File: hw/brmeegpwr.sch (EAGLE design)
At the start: 9 parts, among them IC1 MAX639, IC2 MAX639, IC3 MAX639

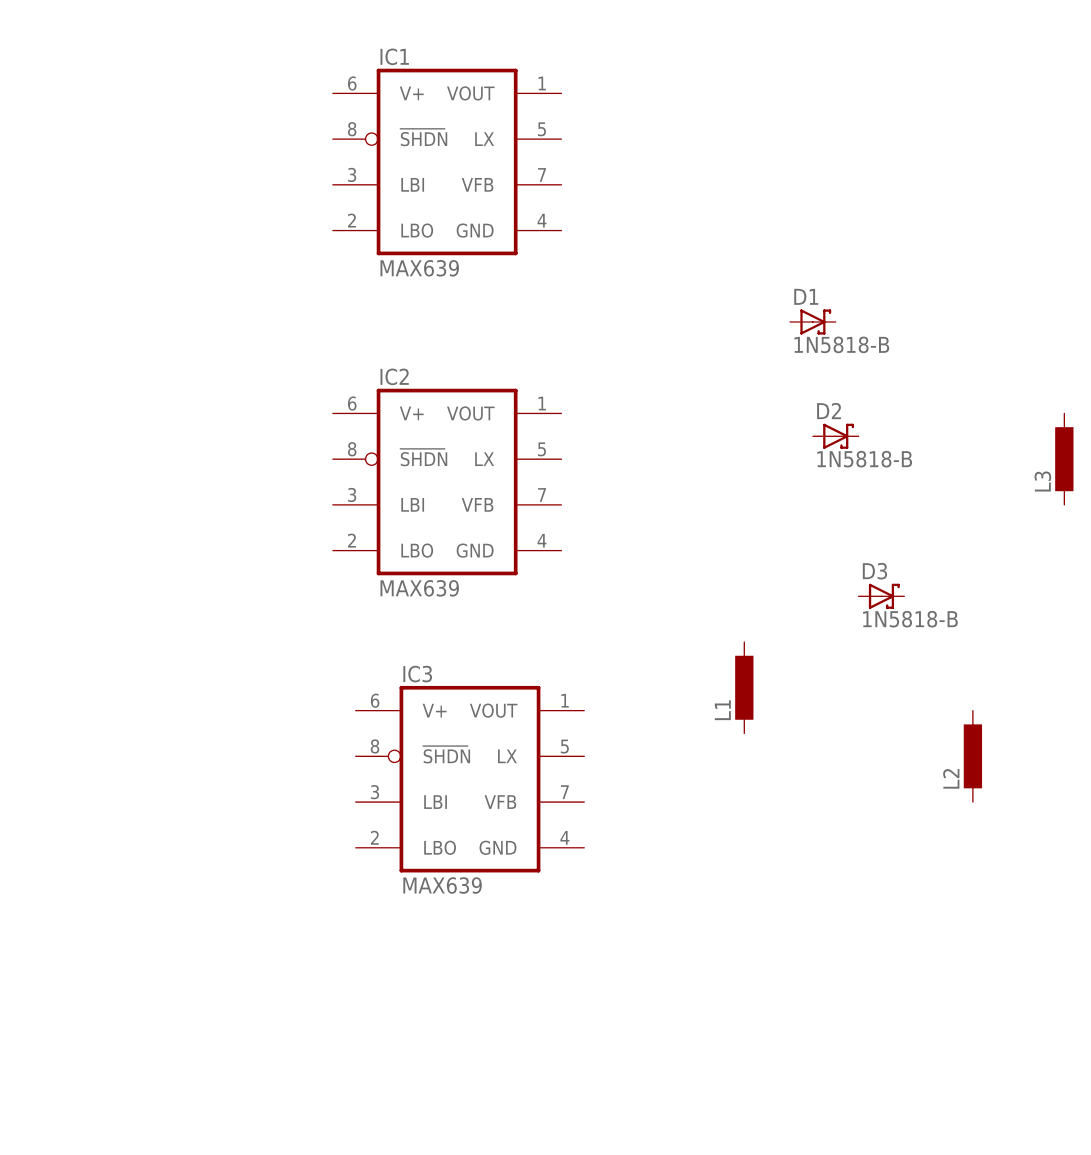
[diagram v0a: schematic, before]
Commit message: power supplies
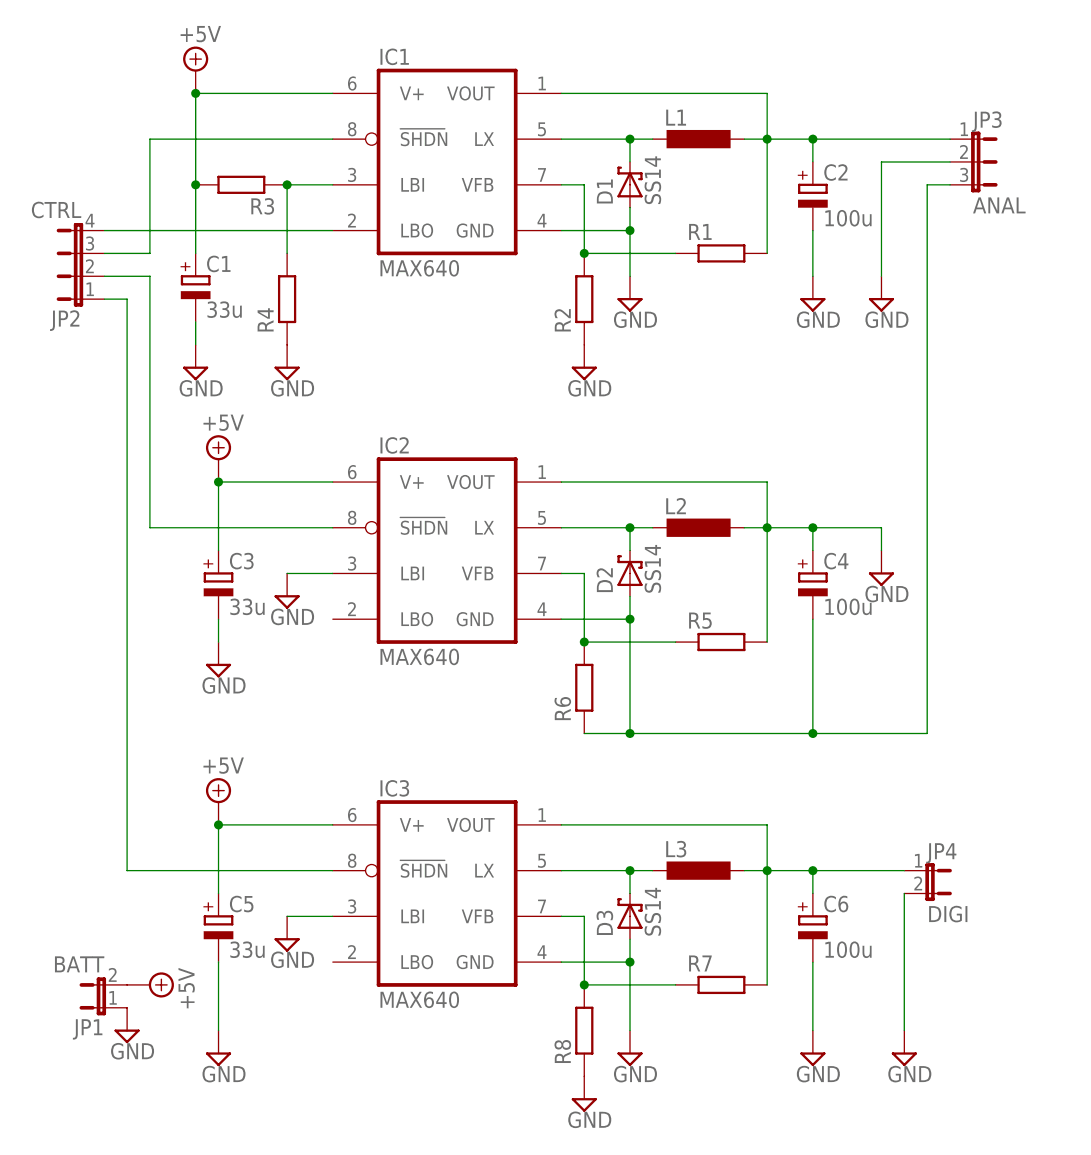
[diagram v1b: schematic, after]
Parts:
- added C1, C3, C5: 33u, rcl:CPOL-EUSMCC
- added C2, C4, C6: 100u, rcl:CPOL-EUSMCC
- added JP1: BATT, jumper:JP1E
- added JP2: CTRL, jumper:JP4E
- added JP3: ANAL, jumper:JP2E
- added JP4: DIGI, jumper:JP1E
- added R1, R2, R3, R4, R5, R6, R7, R8: (no value), rcl:R-EU_R1206
- D1, D2, D3: value 1N5818-B -> SS14; device diode:1N5818-B -> mindspy:SS14
- IC1, IC2, IC3: value MAX639 -> MAX640; device maxim:MAX639 -> mindspy:MAX640
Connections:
- new net +2V5: C2.+, IC1.VOUT, JP3.1, L1.1, R1.2
- new net +5V: C1.+, C3.+, C5.+, IC1.V+, IC2.V+, IC3.V+, JP1.2, R3.2
- new net -2V5: C4.-, D2.A, IC2.GND, JP3.3, R6.1
- new net 3V3: C6.+, IC3.VOUT, JP4.1, L3.1, R7.2
- new net GND: C1.-, C2.-, C3.-, C4.+, C5.-, C6.-, D1.A, D3.A, IC1.GND, IC2.LBI, IC2.VOUT, IC3.GND, IC3.LBI, JP1.1, JP3.2, JP4.2, L2.1, R2.1, R4.1, R5.2, R8.1
- new net N$1: D1.C, IC1.LX, L1.2
- new net N$10: IC2.VFB, R5.1, R6.2
- new net N$11: IC2.SHDN, JP2.2
- new net N$13: IC3.VFB, R7.1, R8.2
- new net N$14: IC3.SHDN, JP2.1
- new net N$2: IC1.SHDN, JP2.3
- new net N$3: IC1.LBO, JP2.4
- new net N$4: D2.C, IC2.LX, L2.2
- new net N$6: IC1.LBI, R3.1, R4.2
- new net N$8: IC1.VFB, R1.1, R2.2
- new net N$9: D3.C, IC3.LX, L3.2
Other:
- moved on the sheet: IC2, IC3, L1, L2, L3
